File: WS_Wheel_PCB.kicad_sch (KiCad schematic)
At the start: 6 parts, among them U1 Teensy4.1

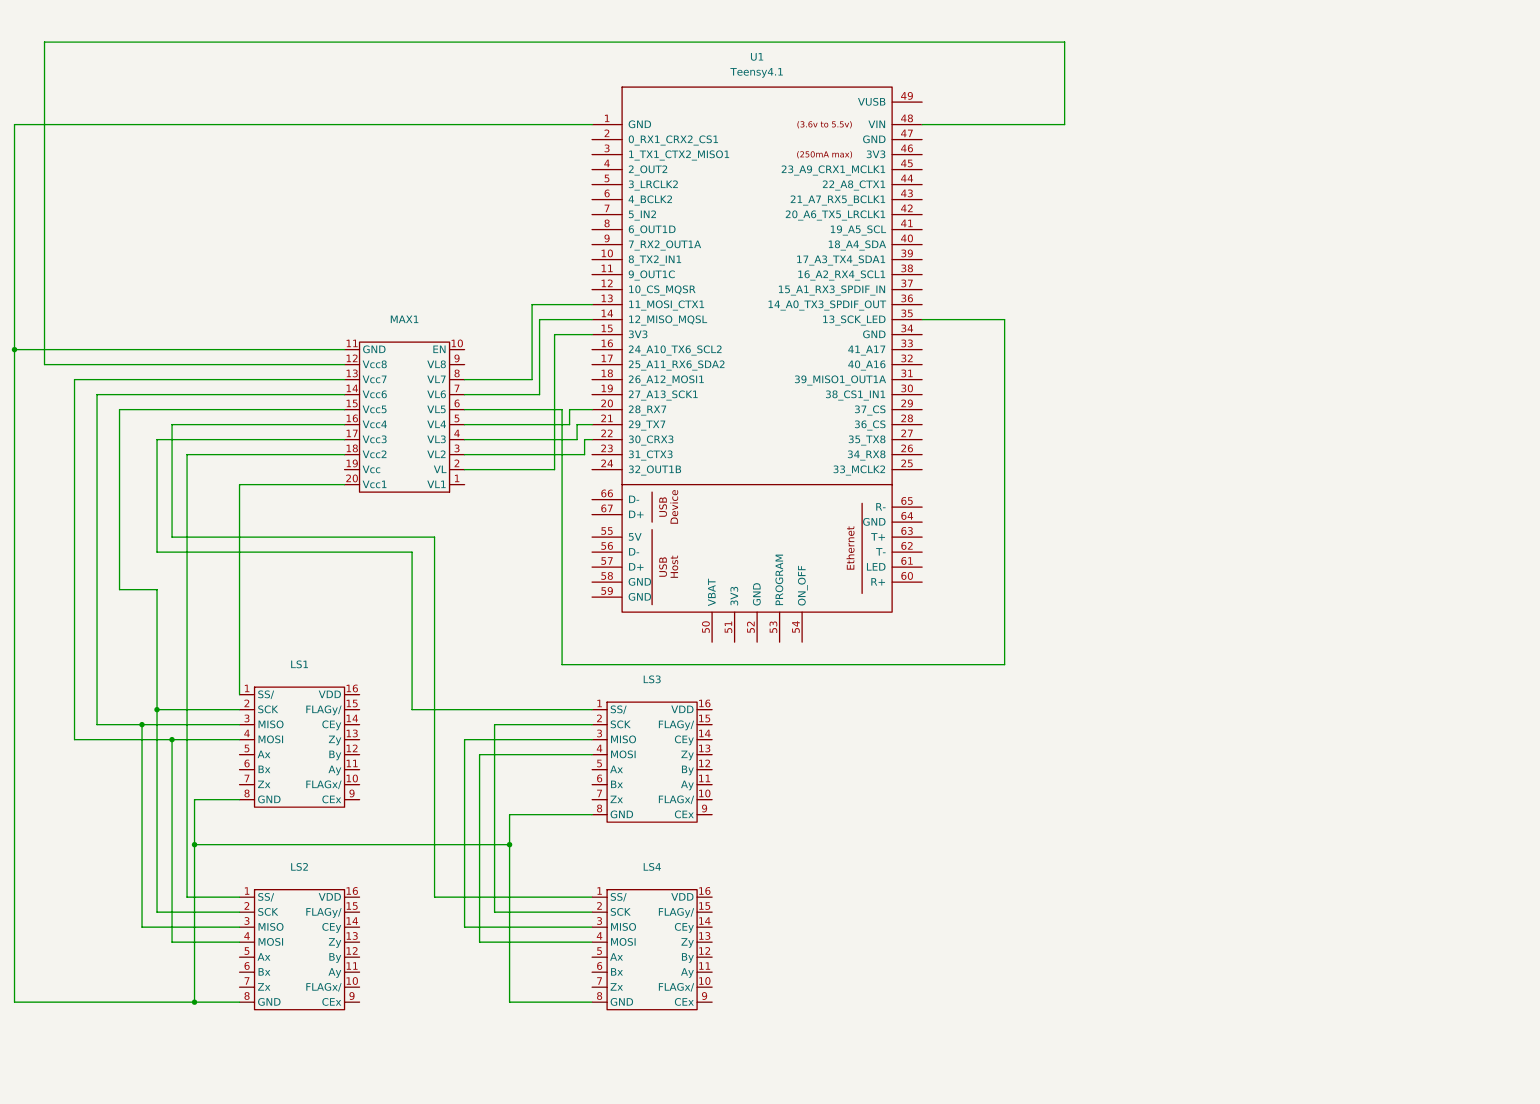
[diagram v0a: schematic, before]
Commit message: Making progress
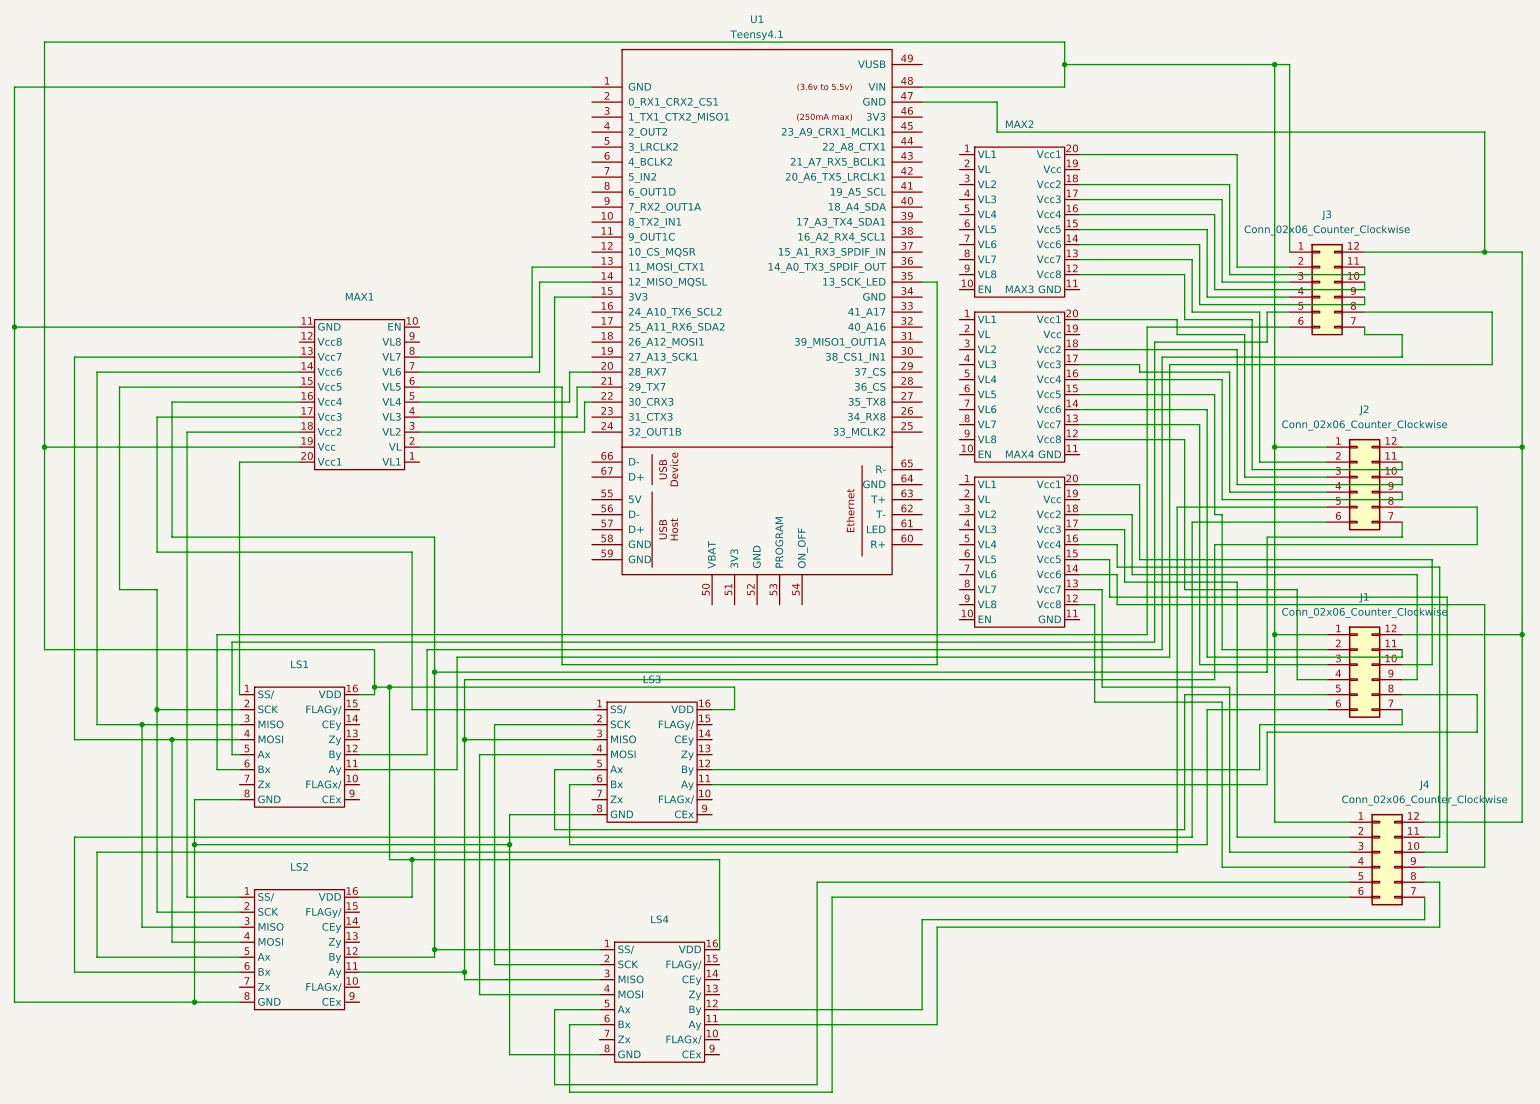
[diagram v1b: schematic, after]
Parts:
- added J1, J2, J3, J4: Conn_02x06_Counter_Clockwise, symbol Connector_Generic:Conn_02x06_Counter_Clockwise
- added MAX2, MAX3, MAX4: ~, Custom_Components:MAX3002, symbol custom_components:MAX3002
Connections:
- net at LS2.11 (Ay): now also LS3.3 (MISO), LS4.3 (MISO), J2.8 (Pin_8)
- net at LS2.12 (By): now also LS4.1 (SS/), MAX1.16 (Vcc4), J2.7 (Pin_7)
- net at LS2.16 (VDD): now also LS1.16 (VDD), LS3.16 (VDD), LS4.16 (VDD), MAX1.19 (Vcc), U1.48 (VIN), J1.1 (Pin_1), J2.1 (Pin_1), J3.1 (Pin_1), J4.1 (Pin_1)
- net at LS2.5 (Ax): now also J2.5 (Pin_5)
- net at LS2.6 (Bx): now also J2.6 (Pin_6)
- net at MAX1.12 (Vcc8): no longer U1.48 (VIN)
- net at LS1.11 (Ay): now also J3.8 (Pin_8)
- net at LS1.12 (By): now also J3.7 (Pin_7)
- net at LS1.5 (Ax): now also J3.5 (Pin_5)
- net at LS1.6 (Bx): now also J3.6 (Pin_6)
- net at LS3.11 (Ay): now also J1.8 (Pin_8)
- net at LS3.12 (By): now also J1.7 (Pin_7)
- net at LS3.5 (Ax): now also J1.5 (Pin_5)
- net at LS3.6 (Bx): now also J1.6 (Pin_6)
- net at U1.47 (GND): now also J1.12 (Pin_12), J2.12 (Pin_12), J3.12 (Pin_12), J4.12 (Pin_12)
- net at LS4.11 (Ay): now also J4.8 (Pin_8)
- net at LS4.12 (By): now also J4.7 (Pin_7)
- net at LS4.5 (Ax): now also J4.5 (Pin_5)
- net at LS4.6 (Bx): now also J4.6 (Pin_6)
- new net: J1.4 (Pin_4), MAX3.12 (Vcc8)
- new net: J1.3 (Pin_3), MAX3.13 (Vcc7)
- new net: J1.11 (Pin_11), MAX3.14 (Vcc6)
- new net: J1.2 (Pin_2), MAX3.15 (Vcc5)
- new net: J2.9 (Pin_9), MAX3.16 (Vcc4)
- new net: J2.4 (Pin_4), MAX3.17 (Vcc3)
- new net: J2.10 (Pin_10), MAX3.18 (Vcc2)
- new net: J2.3 (Pin_3), MAX3.20 (Vcc1)
- new net: J2.11 (Pin_11), MAX2.12 (Vcc8)
- new net: J2.2 (Pin_2), MAX2.13 (Vcc7)
- new net: J3.9 (Pin_9), MAX2.14 (Vcc6)
- new net: J3.4 (Pin_4), MAX2.15 (Vcc5)
- new net: J3.10 (Pin_10), MAX2.16 (Vcc4)
- new net: J3.3 (Pin_3), MAX2.17 (Vcc3)
- new net: J3.11 (Pin_11), MAX2.18 (Vcc2)
- new net: J3.2 (Pin_2), MAX2.20 (Vcc1)
- new net: J4.10 (Pin_10), MAX4.15 (Vcc5)
- new net: J4.11 (Pin_11), MAX4.16 (Vcc4)
- new net: J4.2 (Pin_2), MAX4.17 (Vcc3)
- new net: J4.3 (Pin_3), MAX4.13 (Vcc7)
- new net: J4.4 (Pin_4), MAX4.12 (Vcc8)
- new net: J4.9 (Pin_9), MAX4.14 (Vcc6)
- new net: J1.10 (Pin_10), MAX4.20 (Vcc1)
- new net: J1.9 (Pin_9), MAX4.18 (Vcc2)
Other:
- moved on the sheet: LS4, MAX1, U1
